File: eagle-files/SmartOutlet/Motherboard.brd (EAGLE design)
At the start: 58.4 x 68.2 mm, 35 parts, among them IC1 1117, T1 CST-1025, U1 ADS1115IDGST, U2 ESP-WROOM-32, U3 FT232RL, X1 22-23-2041, X2 22-23-2021

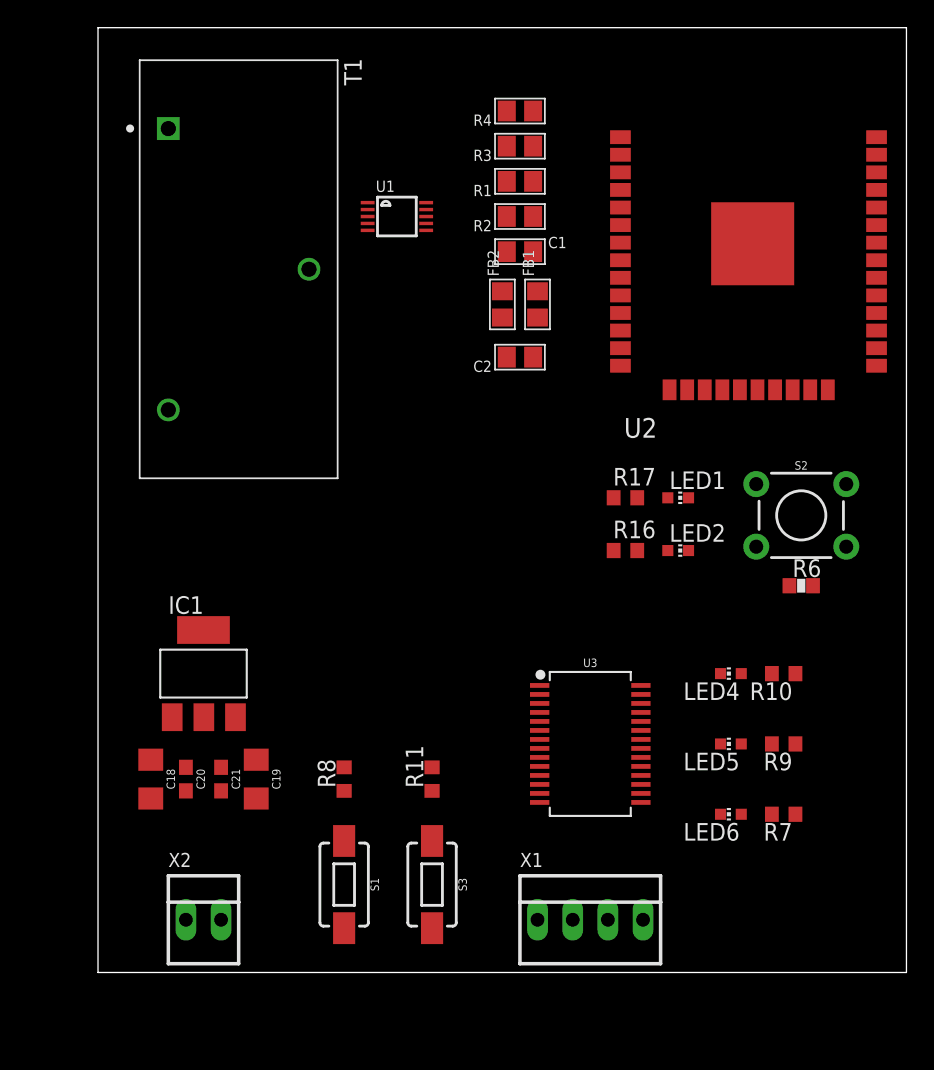
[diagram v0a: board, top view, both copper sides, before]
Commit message: Updated eagle files
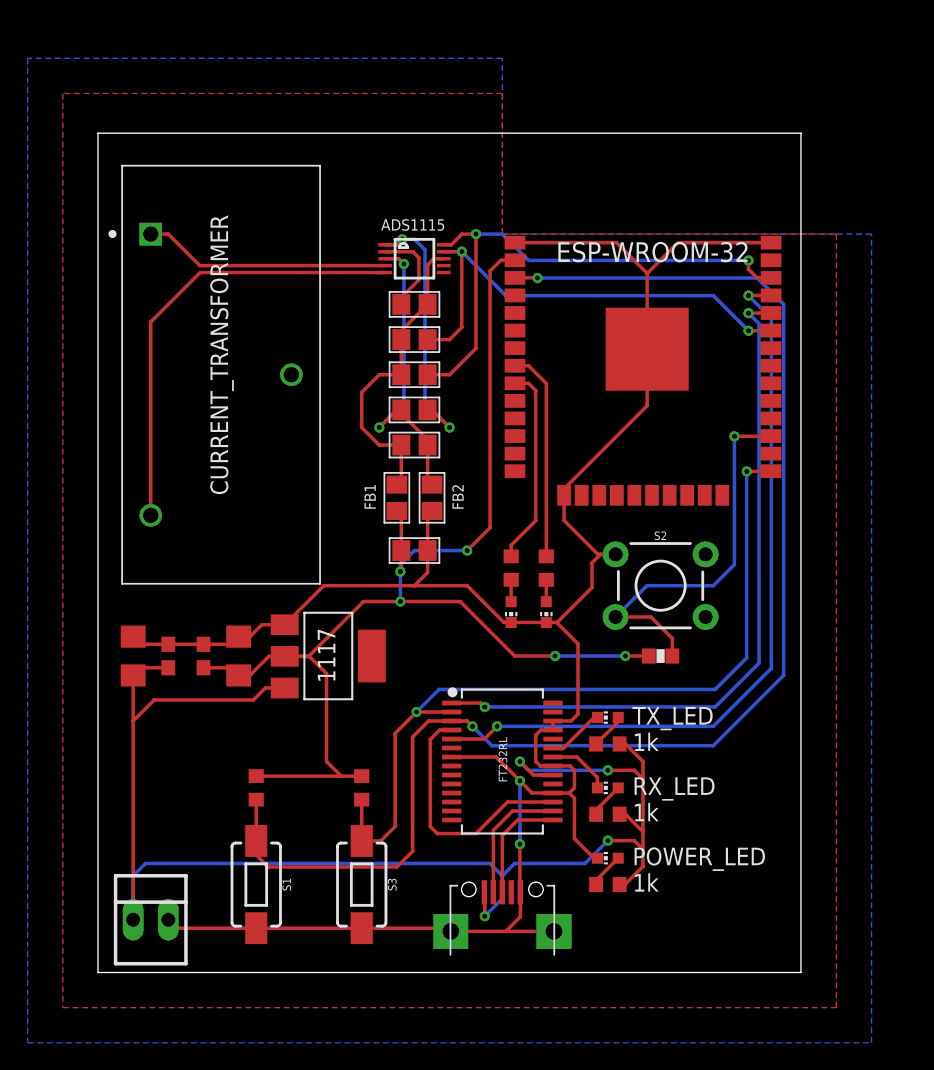
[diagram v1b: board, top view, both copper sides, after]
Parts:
- removed LED4, LED5, LED6: (no value), adafruit:CHIP-LED0603
- removed T1: CST-1025, CST-1025:XFMR_CST-1025
- removed X1: 22-23-2041, con-molex:22-23-2041
- added CURRENT_TRANSFORMER: CST-1025, CST-1025:XFMR_CST-1025
- added POWER_LED, RX_LED, TX_LED: (no value), adafruit:CHIP-LED0603
- added U$1: MICRO-USB, microusb:MICRO-USB
- U1: value ADS1115IDGST -> ADS1115
- moved R3 20.5 mm to (22.9, 40.6), turned to 0 degrees
- moved FB1 17.3 mm to (21.6, 34.3)
- moved C2 15.9 mm to (22.9, 30.5), turned to 0 degrees
- moved C1 15.9 mm to (22.9, 38.1), turned to 180 degrees
- moved R1 15.9 mm to (22.9, 43.2), turned to 0 degrees
- moved R4 15.9 mm to (22.9, 48.3)
- moved FB2 14.9 mm to (24.1, 34.3)
- moved LED1 14.6 mm to (29.8, 26.0), turned to 180 degrees
- moved R9 13.7 mm to (36.8, 11.4)
- moved R10 13.7 mm to (36.8, 16.5)
- moved R7 13.7 mm to (36.8, 6.35)
- moved C19 12.6 mm to (2.54, 22.9), turned to 90 degrees
- moved R2 11.7 mm to (22.9, 45.7), turned to 0 degrees
- moved R6 11.4 mm to (40.6, 22.9), turned to 180 degrees
- moved S2 11.4 mm to (40.6, 27.9)
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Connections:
- net +5V: now also U$1.1, X2.1; no longer X1.1, X2.2
- net BLUE: now also R16.1; no longer R17.1
- net DIFF_INPUT_1: now also CURRENT_TRANSFORMER.1; no longer T1.1
- net DIFF_INPUT_2: now also CURRENT_TRANSFORMER.2; no longer T1.2
- net GND: now also POWER_LED.C, U$1.5, U$1.GND1, U$1.GND2, X2.2; no longer LED6.C, X1.4, X2.1
- net GREEN: now also R17.1; no longer R16.1
- net N$13: now also RX_LED.A; no longer LED5.A
- net N$3: now also TX_LED.A; no longer LED4.A
- net PLUG_D+: now also U$1.3; no longer X1.3
- net PLUG_D-: now also U$1.2; no longer X1.2
- net POWER_LED: now also POWER_LED.A; no longer LED6.A
- net RX_LED: now also RX_LED.C; no longer LED5.C
- net TX_LED: now also TX_LED.C; no longer LED4.C
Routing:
- net GND: track 0.00 -> 166.0 mm, vias 0 -> 2
- net +5V: track 0.00 -> 107.3 mm, vias 0 -> 4
- net RTS: track 0.00 -> 101.5 mm, vias 0 -> 2
- net 3.3V: track 0.00 -> 90.7 mm, vias 0 -> 5
- net DTR: track 0.00 -> 58.0 mm, vias 0 -> 2
- net TX_MCU: track 0.00 -> 54.4 mm, vias 0 -> 2
- net RX_MCU: track 0.00 -> 50.9 mm, vias 0 -> 2
- net SCL: track 0.00 -> 38.2 mm, vias 0 -> 2
- net SDA: track 0.00 -> 34.3 mm, vias 0 -> 2
- net DIFF_INPUT_2: track 0.00 -> 32.4 mm
- net BUTTON: track 0.00 -> 28.1 mm, vias 0 -> 1
- net ADC_GND: track 0.00 -> 22.5 mm, vias 0 -> 2
- net ADC_VCC: track 0.00 -> 22.4 mm
- net ADDR: track 0.00 -> 19.0 mm, vias 0 -> 2
- net 3V3: track 0.00 -> 18.1 mm
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- added copper zone on layer 1, net GND
- added copper zone on layer 16, net GND
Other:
- board size 58.4 x 68.2 mm -> 50.8 x 60.6 mm
